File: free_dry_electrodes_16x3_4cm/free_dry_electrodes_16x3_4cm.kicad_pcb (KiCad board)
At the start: 2 copper layers, 39.6 x 34.3 mm, 27 parts, among them J1 Conn_01x03, J10 Conn_01x03, J11 Conn_01x03, J12 Conn_01x03, J13 Conn_01x03, J14 Conn_01x03, J15 Conn_01x03, J16 Conn_01x03, J17 Conn_01x03, J18 Conn_01x03, J19 Conn_01x03, J2 Conn_01x03, J20 Conn_01x03, J21 Conn_01x03, J22 Conn_01x03, J23 Conn_01x03, J24 Conn_01x03, J3 Conn_01x03, J4 Conn_01x03, J5 Conn_01x03, J6 Conn_01x03, J7 Conn_01x03, J8 Conn_01x03, J9 Conn_01x03

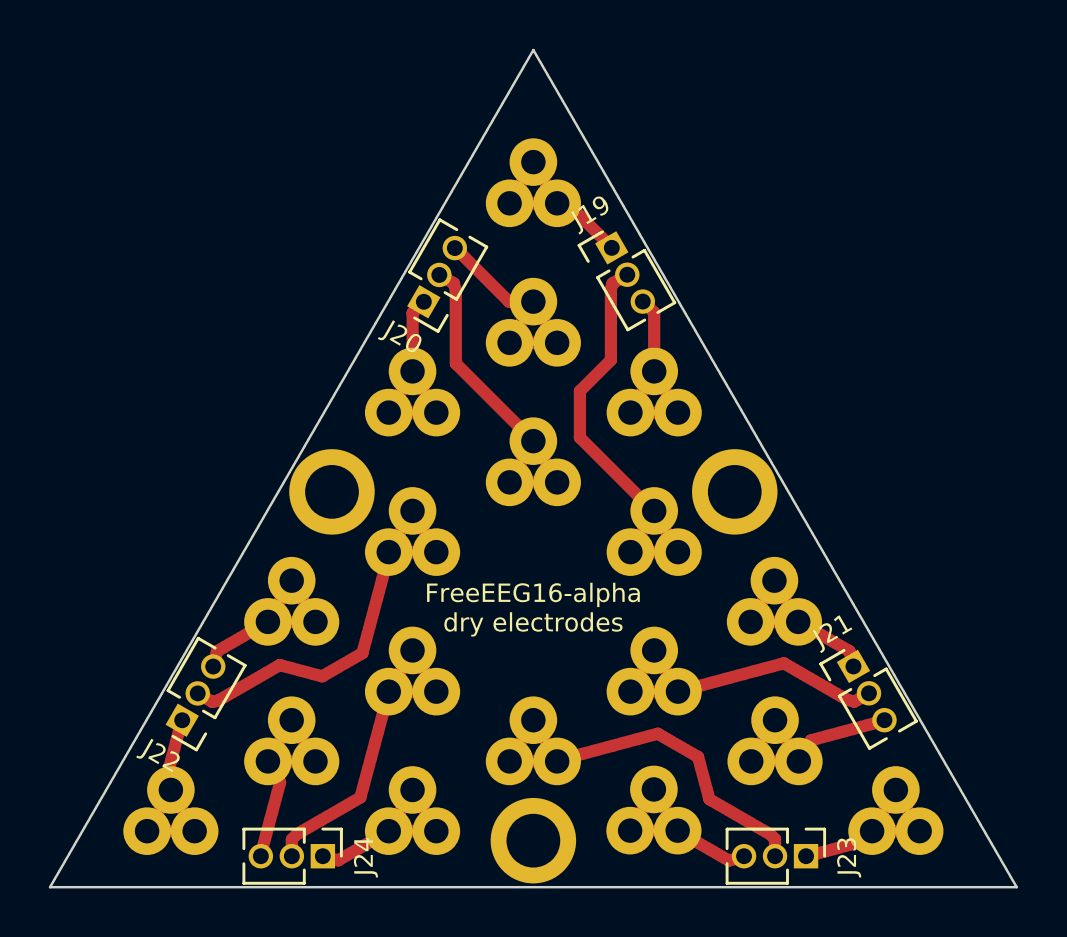
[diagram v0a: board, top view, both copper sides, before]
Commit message: Add files via upload
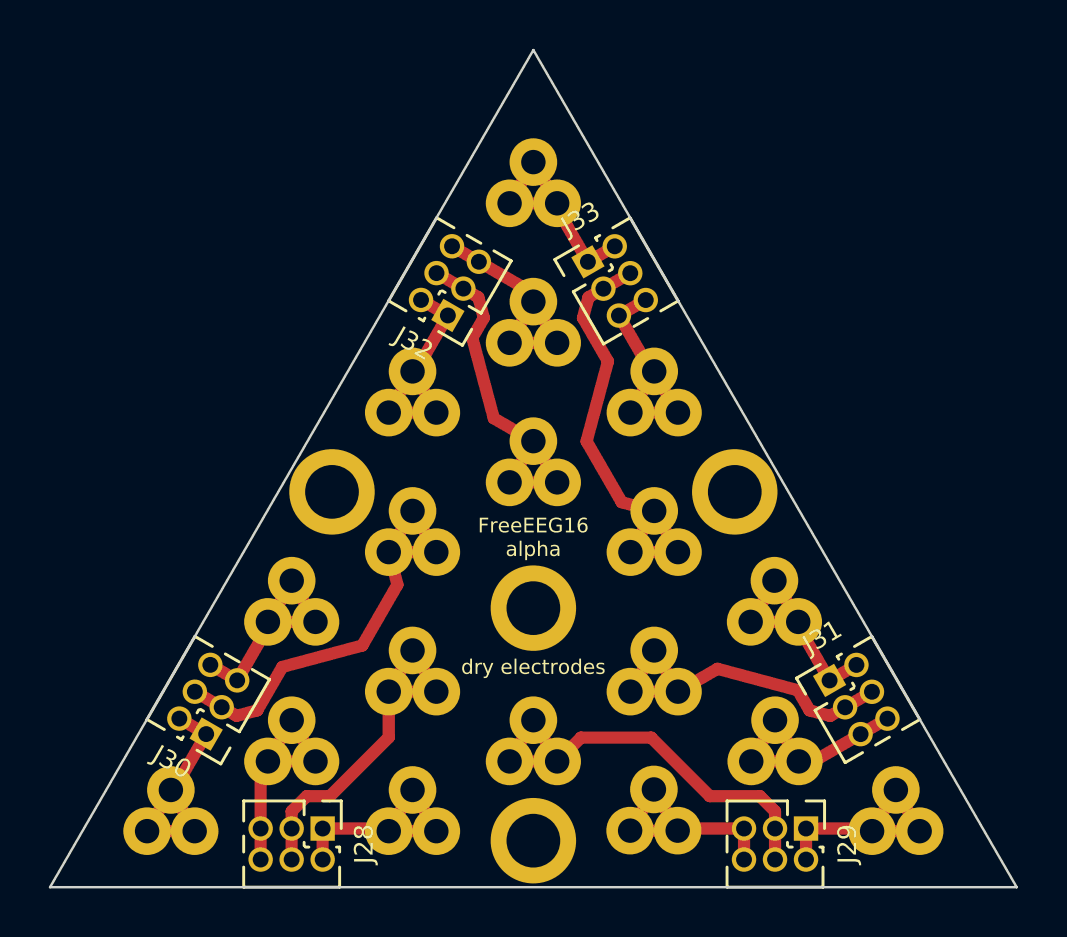
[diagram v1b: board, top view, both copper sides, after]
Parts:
- removed J19, J20, J21, J22, J23, J24: Conn_01x03, Connector_PinHeader_1.27mm:PinHeader_1x03_P1.27mm_Vertical
- added J28: Conn_02x03_Odd_Even, Connector_PinHeader_1.27mm:PinHeader_2x03_P1.27mm_Vertical, F.Cu at (-8.63, 9.03)
- added J29: Conn_02x03_Odd_Even, Connector_PinHeader_1.27mm:PinHeader_2x03_P1.27mm_Vertical, F.Cu at (11.2, 9.03)
- added J30: Conn_02x03_Odd_Even, Connector_PinHeader_1.27mm:PinHeader_2x03_P1.27mm_Vertical, F.Cu at (-13.4, 5.16)
- added J31: Conn_02x03_Odd_Even, Connector_PinHeader_1.27mm:PinHeader_2x03_P1.27mm_Vertical, F.Cu at (12.1, 2.96)
- added J32: Conn_02x03_Odd_Even, Connector_PinHeader_1.27mm:PinHeader_2x03_P1.27mm_Vertical, F.Cu at (-3.50, -12.0)
- added J33: Conn_02x03_Odd_Even, Connector_PinHeader_1.27mm:PinHeader_2x03_P1.27mm_Vertical, F.Cu at (2.23, -14.2)
- added REF**: MountingHole_2.2mm_M2_ISO7380_Pad, MountingHole:MountingHole_2.2mm_M2_ISO7380_Pad, F.Cu at (0.00, 0.00)
- J1, J10, J11, J12, J13, J14, J15, J16, J17, J18, J2, J3, J4, J5, J6, J7, J8, J9: footprint freeeeg16:CPA_3_od4.5_d1.95_id1.0 -> FreeEEG16-alpha:CPA_3_od4.5_d1.95_id1.0
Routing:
- net /J13: track 8.80 -> 9.87 mm
- net /J16: track 8.80 -> 9.87 mm
- net /J1: track 8.80 -> 9.87 mm
- net /J7: track 8.91 -> 9.87 mm
- net /J15: track 8.91 -> 9.87 mm
- net /J4: track 8.91 -> 9.87 mm
- net /J14: track 8.95 -> 9.87 mm
- net /J9: track 8.95 -> 9.87 mm
- net /J3: track 8.95 -> 9.87 mm
- net /J11: track 17.7 -> 18.4 mm
- net /J6: track 17.7 -> 18.4 mm
- net /J5: track 17.7 -> 18.4 mm
- net /J18: track 14.3 -> 14.9 mm
- net /J17: track 14.3 -> 14.9 mm
- net /J8: track 14.3 -> 14.9 mm
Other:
- board text added: "FreeEEG16 alpha dry electrodes"
- board text removed: "FreeEEG16-alpha dry electrodes"
